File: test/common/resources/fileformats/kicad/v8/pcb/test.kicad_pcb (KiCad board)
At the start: 2 copper layers, 4 parts

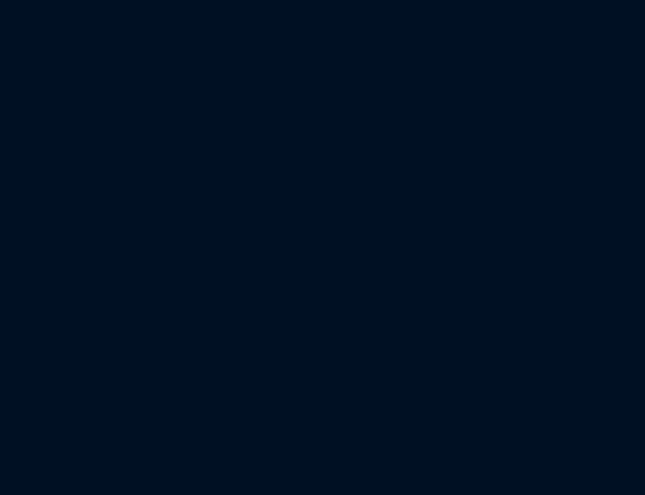
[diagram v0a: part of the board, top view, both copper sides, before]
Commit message: bug fix
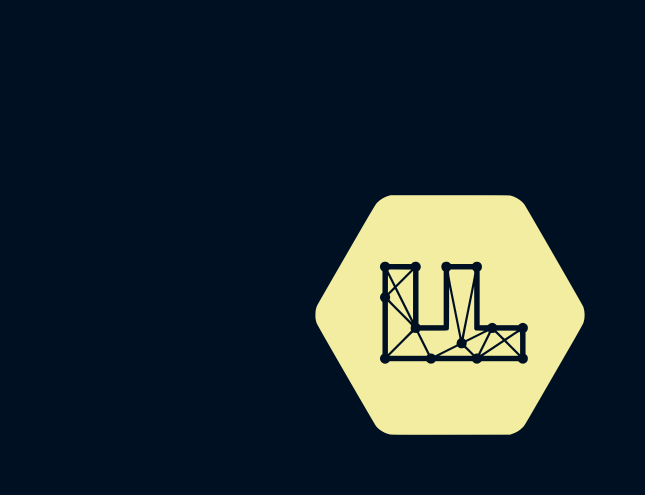
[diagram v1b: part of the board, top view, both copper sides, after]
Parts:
- G***: moved to F.Cu
- moved G*** 22.4 mm to (90.0, 180.0), turned to 90 degrees

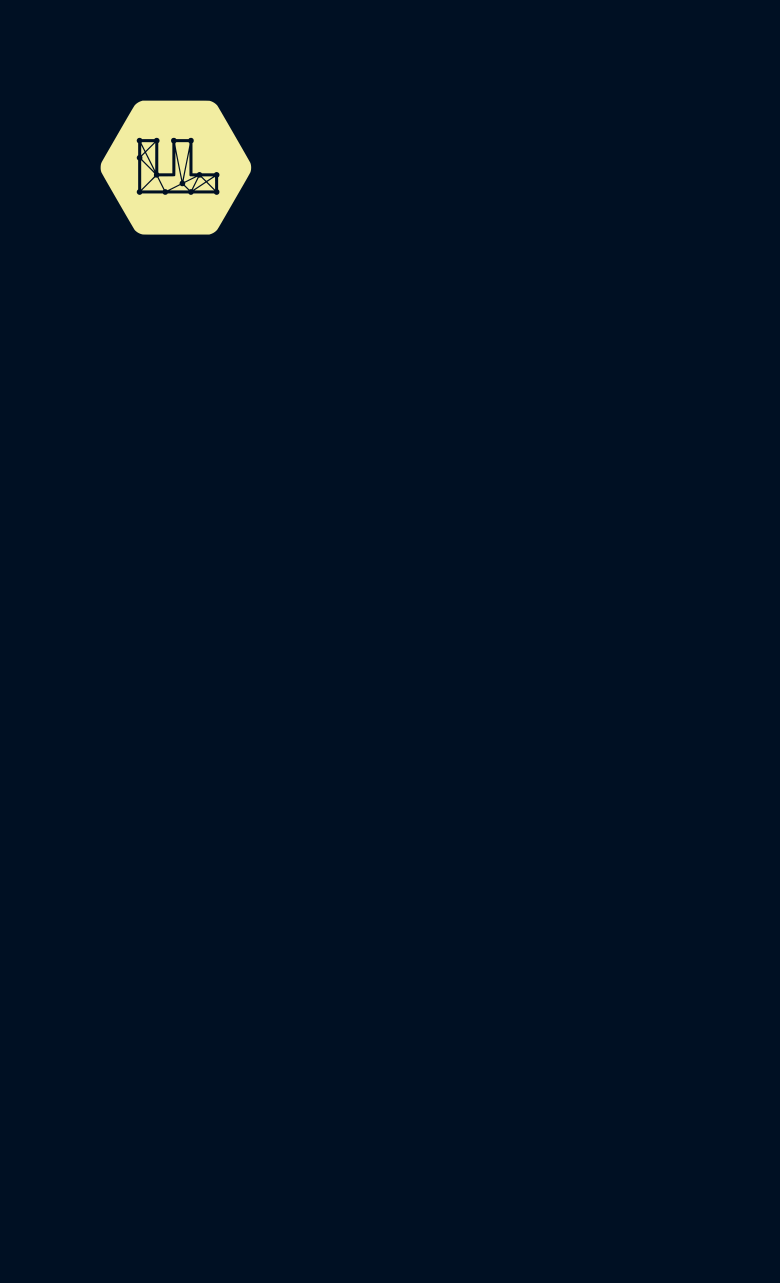
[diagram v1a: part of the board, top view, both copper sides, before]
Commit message: pytest fixes
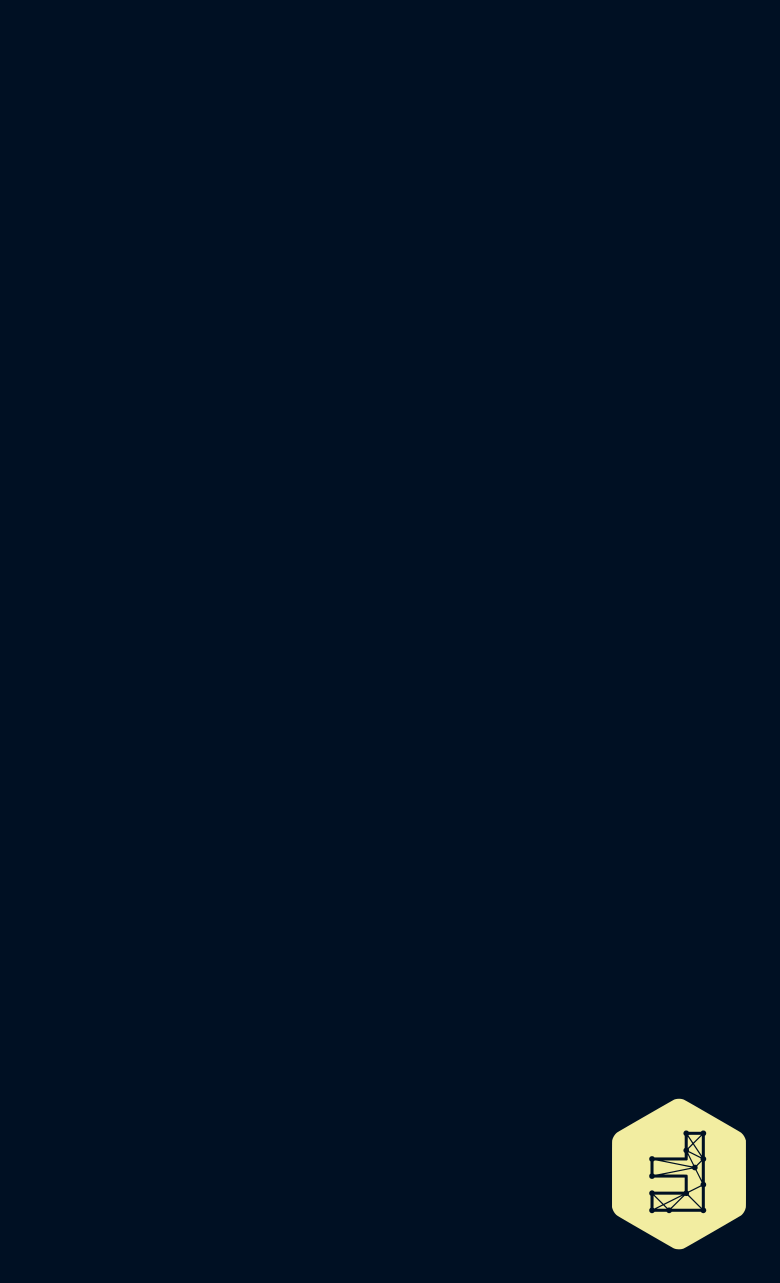
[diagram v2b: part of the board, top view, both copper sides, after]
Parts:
- moved G*** 67.1 mm to (120.0, 240.0), turned to 180 degrees
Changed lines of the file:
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@@
 	(footprint "logos:faebryk_logo"
 		(layer "F.Cu")
-		(at 90 180 90)
+		(at 120 240 180)
 		(property "Reference" "G***"
-			(at 0 0 270)
+			(at 0 0 180)
 			(layer "F.SilkS")
 			(hide yes)
@@
 		)
 		(property "Value" "LOGO"
-			(at 0.75 0 270)
+			(at 0.75 0 180)
 			(layer "F.SilkS")
 			(hide yes)
@@
 		)
 		(property "Footprint" "logos:faebryk_logo"
-			(at 0 0 270)
+			(at 0 0 180)
 			(layer "F.Fab")
 			(hide no)
@@
 		)
 		(property "Datasheet" ""
-			(at 0 0 270)
+			(at 0 0 180)
 			(layer "F.Fab")
 			(hide yes)
@@
 		)
 		(property "Description" ""
-			(at 0 0 270)
+			(at 0 0 180)
 			(layer "F.Fab")
 			(hide yes)

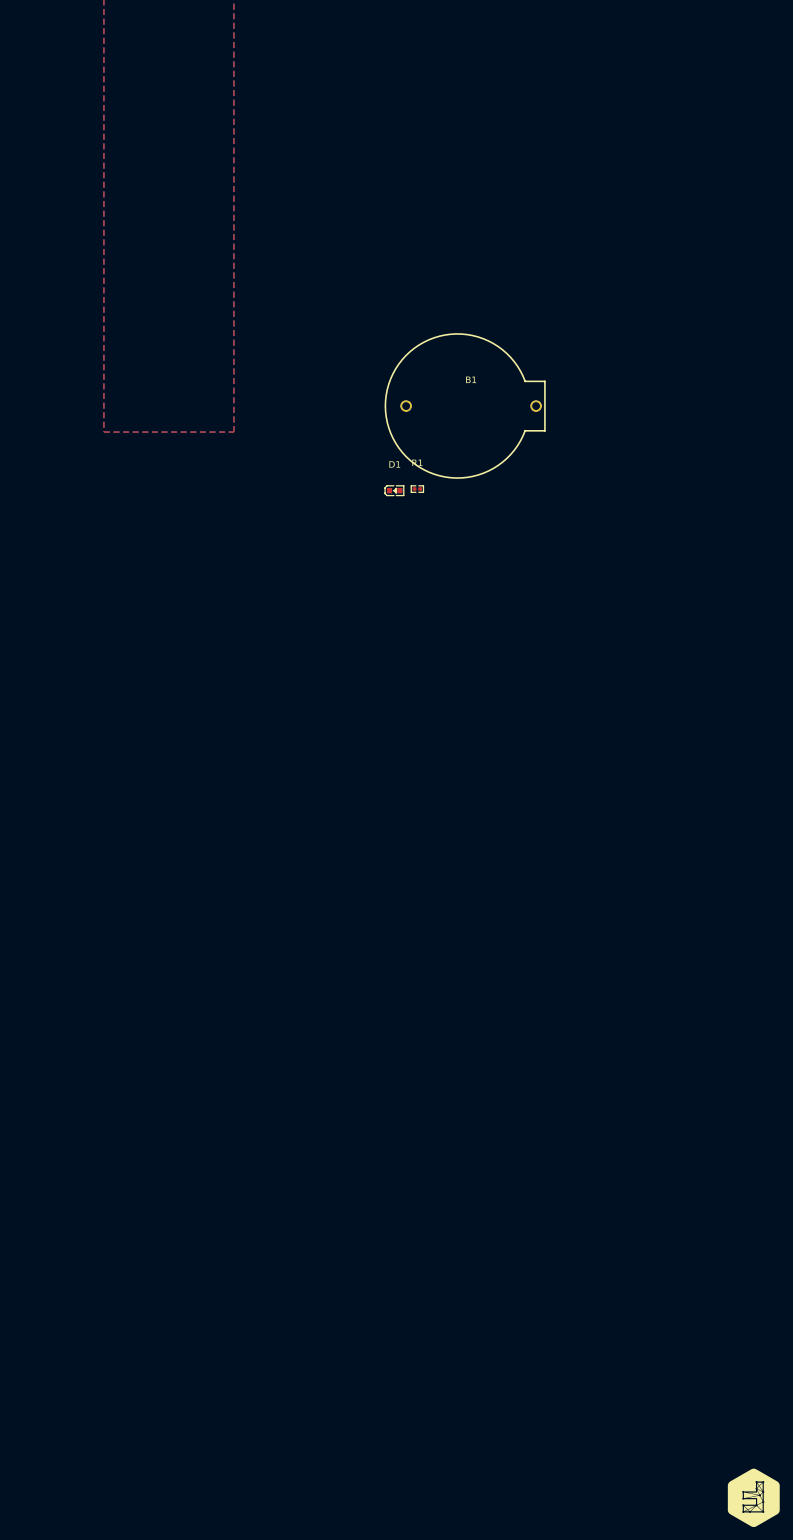
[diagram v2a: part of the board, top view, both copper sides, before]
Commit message: more pytest fix
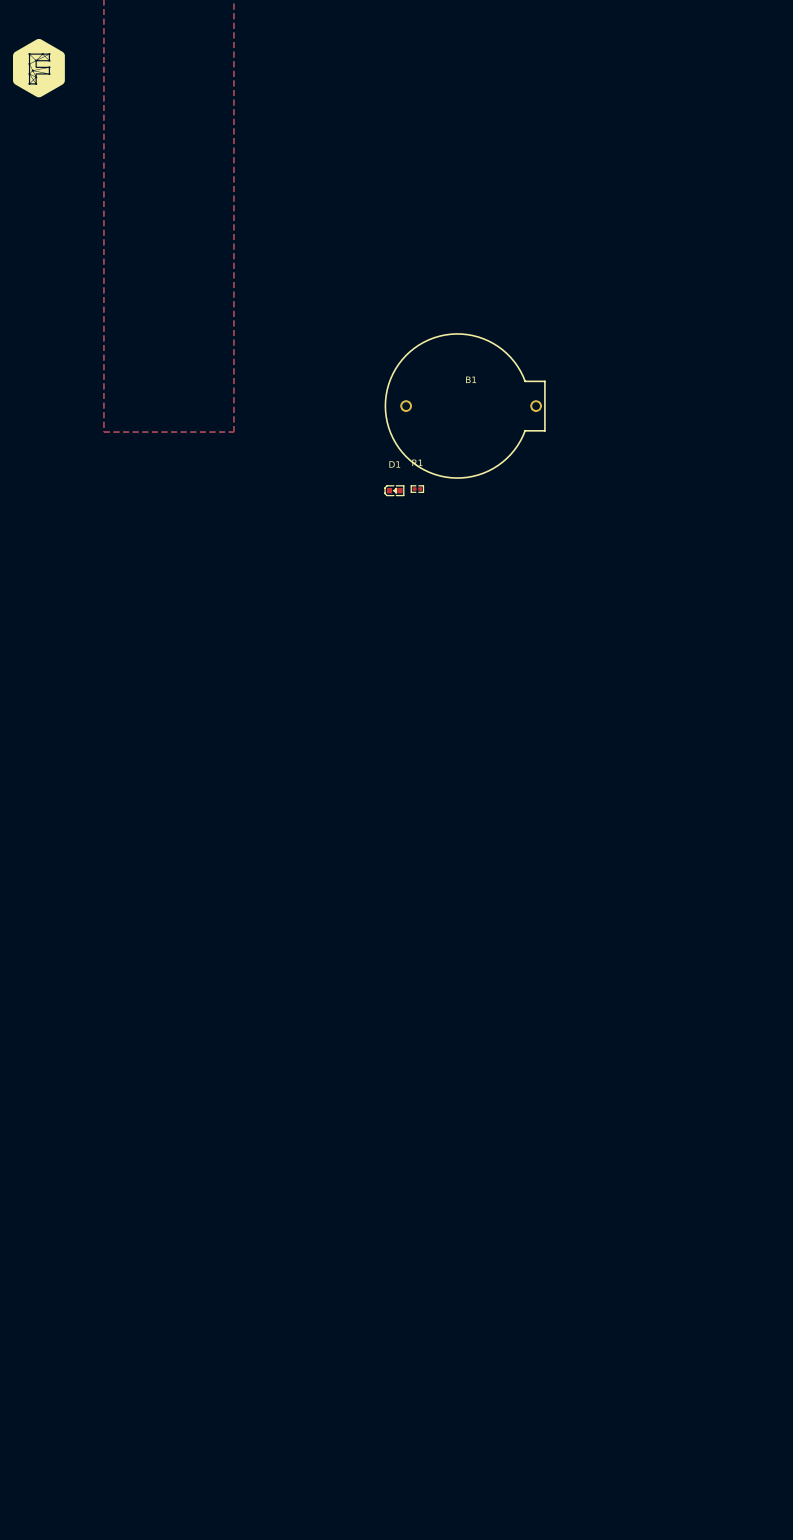
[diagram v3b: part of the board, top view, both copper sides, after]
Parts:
- moved G*** 246.0 mm to (10.0, 20.0), turned to 0 degrees
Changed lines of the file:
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@@
 	(footprint "logos:faebryk_logo"
 		(layer "F.Cu")
-		(at 120 240 180)
+		(at 10 20 0)
 		(property "Reference" "G***"
-			(at 0 0 180)
+			(at 0 0 0)
 			(layer "F.SilkS")
 			(hide yes)
@@
 		)
 		(property "Value" "LOGO"
-			(at 0.75 0 180)
+			(at 0.75 0 0)
 			(layer "F.SilkS")
 			(hide yes)
@@
 		)
 		(property "Footprint" "logos:faebryk_logo"
-			(at 0 0 180)
+			(at 0 0 0)
 			(layer "F.Fab")
 			(hide no)
@@
 					(thickness 0.15)
 				)
-				(justify right mirror)
+				(justify mirror right)
 			)
 		)
 		(property "Datasheet" ""
-			(at 0 0 180)
+			(at 0 0 0)
 			(layer "F.Fab")
 			(hide yes)
@@
 		)
 		(property "Description" ""
-			(at 0 0 180)
+			(at 0 0 0)
 			(layer "F.Fab")
 			(hide yes)
